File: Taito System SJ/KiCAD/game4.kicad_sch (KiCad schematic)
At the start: 21 parts, among them U44 74LS74, U46 74LS74, U56 74LS273, U66 74LS32, U66 74LS367, U67 82S09, U68 74LS08

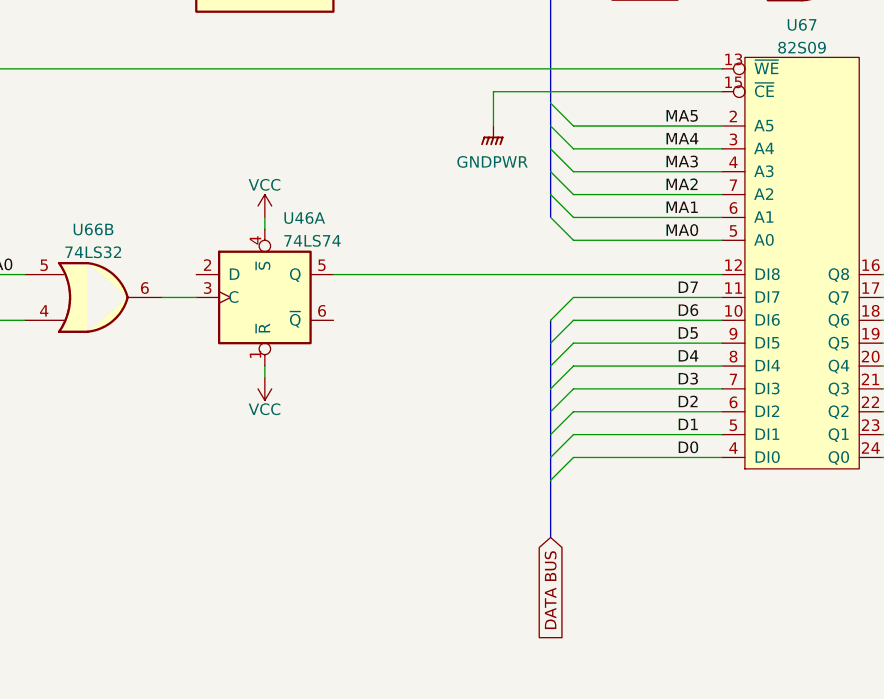
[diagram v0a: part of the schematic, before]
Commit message: Multiple updates while coding core
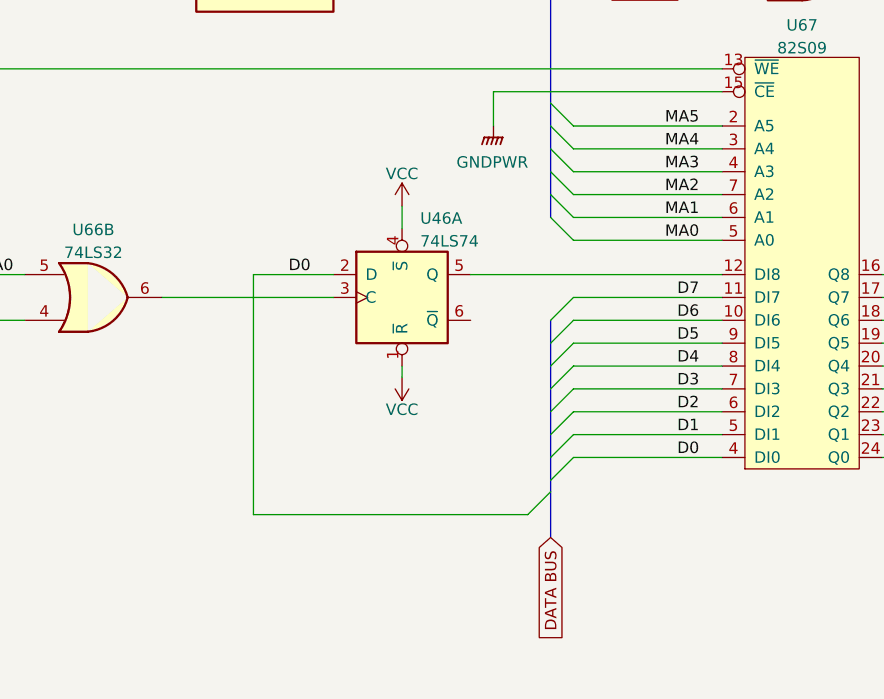
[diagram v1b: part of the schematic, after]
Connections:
- net D0: now also U46.2 (D)
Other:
- moved on the sheet: U46A
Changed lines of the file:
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@@
+    (stroke (width 0) (type default))
+  )
+  (bus_entry (at 129.54 116.84) (size -2.54 2.54)
     (stroke (width 0) (type default))
   )
@@
     (stroke (width 0) (type default))
   )
-  (wire (pts (xy 97.79 104.14) (xy 97.79 102.87))
+  (wire (pts (xy 113.03 104.14) (xy 113.03 102.87))
     (stroke (width 0) (type default))
   )
@@
     (stroke (width 0) (type default))
   )
+  (wire (pts (xy 96.52 92.71) (xy 96.52 119.38))
+    (stroke (width 0) (type default))
+  )
   (bus (pts (xy 129.54 53.34) (xy 129.54 55.88))
     (stroke (width 0) (type default))
@@
     (stroke (width 0) (type default))
   )
-  (wire (pts (xy 86.36 95.25) (xy 90.17 95.25))
+  (wire (pts (xy 86.36 95.25) (xy 105.41 95.25))
     (stroke (width 0) (type default))
   )
@@
     (stroke (width 0) (type default))
   )
-  (wire (pts (xy 97.79 86.36) (xy 97.79 87.63))
+  (wire (pts (xy 113.03 85.09) (xy 113.03 87.63))
     (stroke (width 0) (type default))
   )
@@
     (stroke (width 0) (type default))
   )
+  (wire (pts (xy 105.41 92.71) (xy 96.52 92.71))
+    (stroke (width 0) (type default))
+  )
   (bus (pts (xy 129.54 45.72) (xy 129.54 48.26))
     (stroke (width 0) (type default))
@@
     (stroke (width 0) (type default))
   )
-  (wire (pts (xy 105.41 92.71) (xy 148.59 92.71))
+  (wire (pts (xy 120.65 92.71) (xy 148.59 92.71))
     (stroke (width 0) (type default))
   )
@@
     (stroke (width 0) (type default))
   )
-  (bus (pts (xy 129.54 115.57) (xy 129.54 121.92))
+  (bus (pts (xy 129.54 115.57) (xy 129.54 116.84))
     (stroke (width 0) (type default))
   )
@@
     (stroke (width 0) (type default))
   )
+  (bus (pts (xy 129.54 116.84) (xy 129.54 121.92))
+    (stroke (width 0) (type default))
+  )
   (wire (pts (xy 214.63 95.25) (xy 228.6 95.25))
     (stroke (width 0) (type default))
@@
     (stroke (width 0) (type default))
   )
+  (wire (pts (xy 96.52 119.38) (xy 127 119.38))
+    (stroke (width 0) (type default))
+  )
   (wire (pts (xy 148.59 72.39) (xy 123.19 72.39))
     (stroke (width 0) (type default))
@@
   )
   (label "A0" (at 69.85 92.71 180) (fields_autoplaced)
+    (effects (font (size 1.27 1.27)) (justify right bottom))
+  )
+  (label "D0" (at 102.87 92.71 180) (fields_autoplaced)
     (effects (font (size 1.27 1.27)) (justify right bottom))
   )
@@
     )
   )
-  (symbol (lib_id "power:VCC") (at 97.79 104.14 0) (mirror x) (unit 1)
-    (in_bom yes) (on_board yes) (dnp no) (fields_autoplaced)
-    (property "Reference" "#PWR?" (at 97.79 100.33 0)
-      (effects (font (size 1.27 1.27)) hide)
-    )
-    (property "Value" "VCC" (at 97.79 107.7158 0)
+  (symbol (lib_id "power:VCC") (at 113.03 104.14 0) (mirror x) (unit 1)
+    (in_bom yes) (on_board yes) (dnp no) (fields_autoplaced)
+    (property "Reference" "#PWR?" (at 113.03 100.33 0)
+      (effects (font (size 1.27 1.27)) hide)
+    )
+    (property "Value" "VCC" (at 113.03 107.7158 0)
       (effects (font (size 1.27 1.27)))
     )
-    (property "Footprint" "" (at 97.79 104.14 0)
-      (effects (font (size 1.27 1.27)) hide)
-    )
-    (property "Datasheet" "" (at 97.79 104.14 0)
+    (property "Footprint" "" (at 113.03 104.14 0)
+      (effects (font (size 1.27 1.27)) hide)
+    )
+    (property "Datasheet" "" (at 113.03 104.14 0)
       (effects (font (size 1.27 1.27)) hide)
     )
@@
     )
   )
-  (symbol (lib_id "power:VCC") (at 97.79 86.36 0) (unit 1)
-    (in_bom yes) (on_board yes) (dnp no) (fields_autoplaced)
-    (property "Reference" "#PWR?" (at 97.79 90.17 0)
-      (effects (font (size 1.27 1.27)) hide)
-    )
-    (property "Value" "VCC" (at 97.79 82.7842 0)
+  (symbol (lib_id "power:VCC") (at 113.03 85.09 0) (unit 1)
+    (in_bom yes) (on_board yes) (dnp no) (fields_autoplaced)
+    (property "Reference" "#PWR?" (at 113.03 88.9 0)
+      (effects (font (size 1.27 1.27)) hide)
+    )
+    (property "Value" "VCC" (at 113.03 81.5142 0)
       (effects (font (size 1.27 1.27)))
     )
-    (property "Footprint" "" (at 97.79 86.36 0)
-      (effects (font (size 1.27 1.27)) hide)
-    )
-    (property "Datasheet" "" (at 97.79 86.36 0)
+    (property "Footprint" "" (at 113.03 85.09 0)
+      (effects (font (size 1.27 1.27)) hide)
+    )
+    (property "Datasheet" "" (at 113.03 85.09 0)
       (effects (font (size 1.27 1.27)) hide)
     )
@@
     )
   )
-  (symbol (lib_id "jt74:74LS74") (at 97.79 95.25 0) (unit 1)
-    (in_bom yes) (on_board yes) (dnp no) (fields_autoplaced)
-    (property "Reference" "U46" (at 99.8094 86.4702 0)
+  (symbol (lib_id "jt74:74LS74") (at 113.03 95.25 0) (unit 1)
+    (in_bom yes) (on_board yes) (dnp no) (fields_autoplaced)
+    (property "Reference" "U46" (at 115.0494 86.4702 0)
       (effects (font (size 1.27 1.27)) (justify left))
     )
-    (property "Value" "74LS74" (at 99.8094 89.0071 0)
+    (property "Value" "74LS74" (at 115.0494 89.0071 0)
       (effects (font (size 1.27 1.27)) (justify left))
     )
-    (property "Footprint" "" (at 97.79 95.25 0)
-      (effects (font (size 1.27 1.27)) hide)
-    )
-    (property "Datasheet" "74xx/74hc_hct74.pdf" (at 97.79 95.25 0)
-      (effects (font (size 1.27 1.27)) hide)
-    )
+    (property "Footprint" "" (at 113.03 95.25 0)
+      (effects (font (size 1.27 1.27)) hide)
+    )
+    (property "Datasheet" "74xx/74hc_hct74.pdf" (at 113.03 95.25 0)
+      (effects (font (size 1.27 1.27)) hide)
+    )
